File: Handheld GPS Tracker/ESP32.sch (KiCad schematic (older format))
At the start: 27 parts

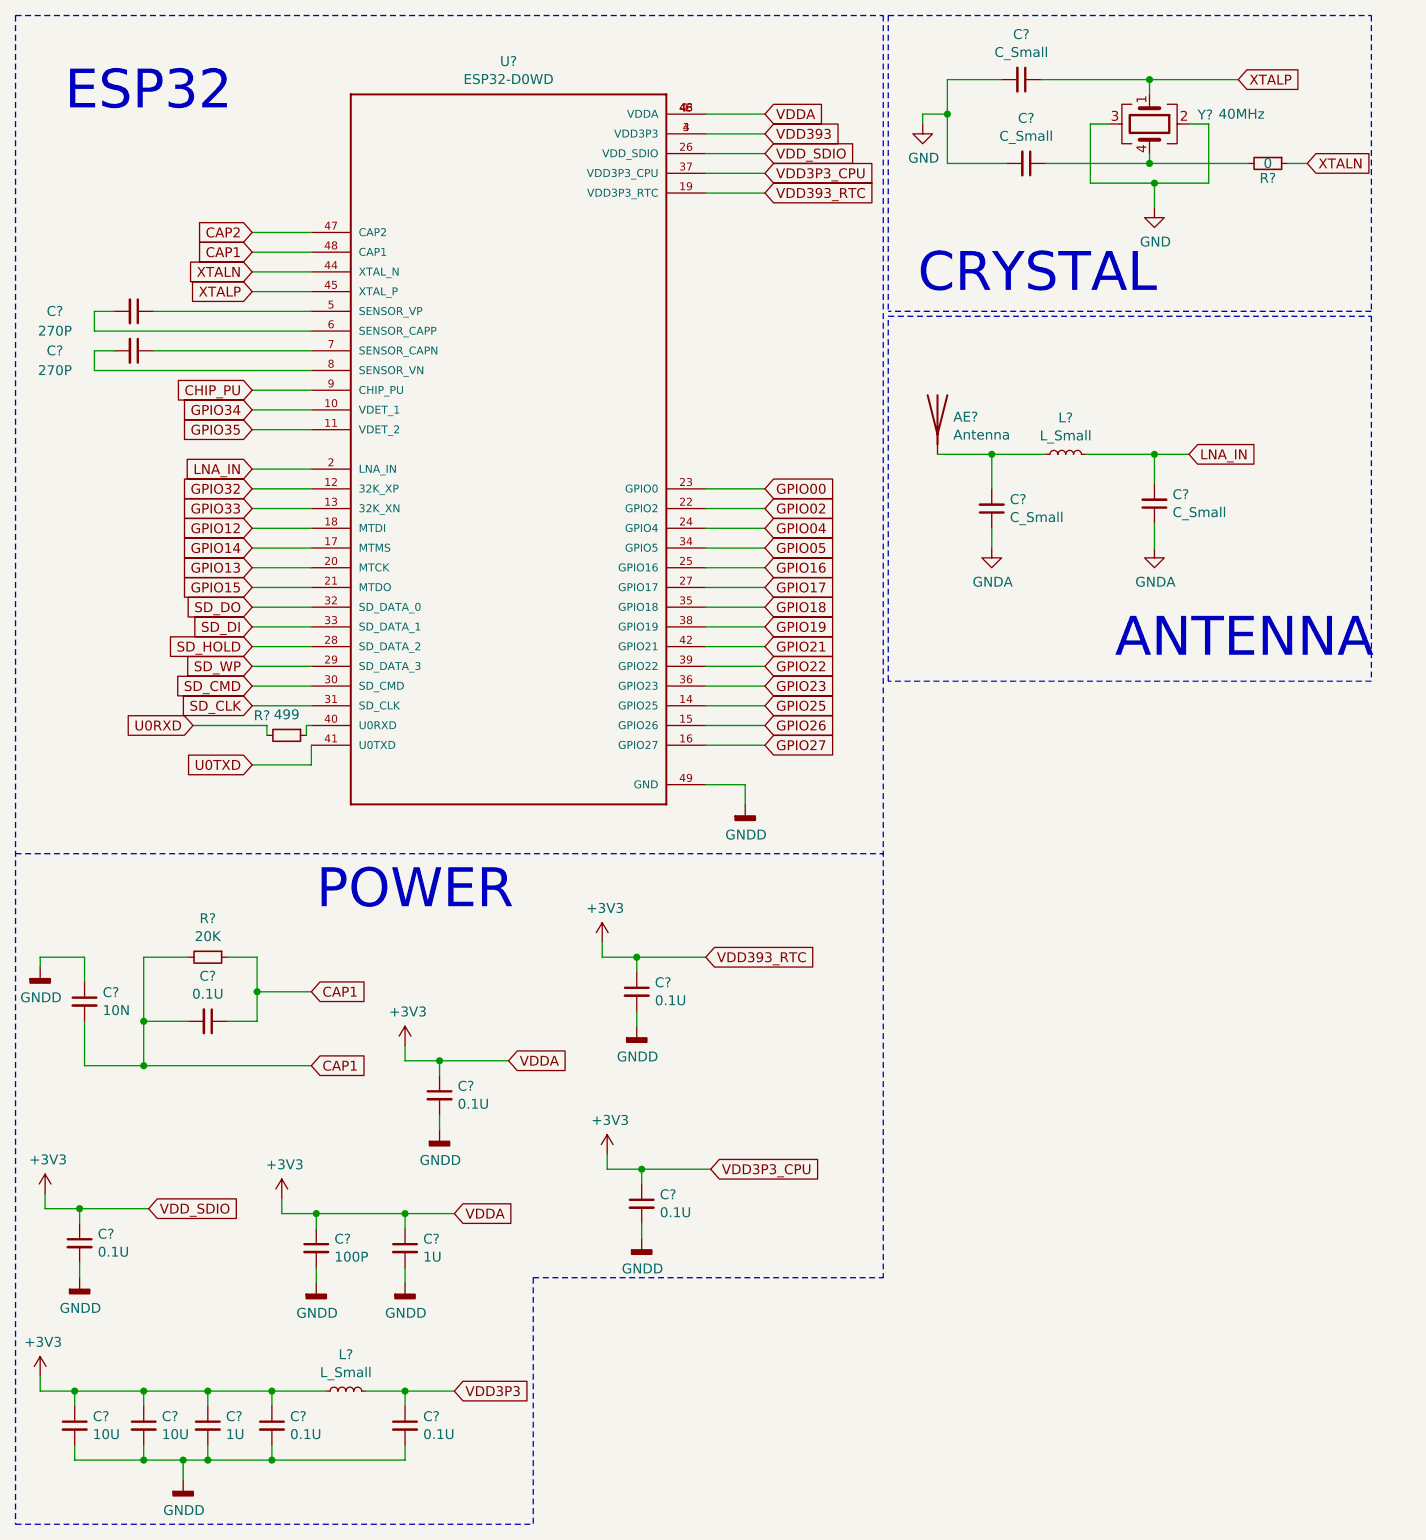
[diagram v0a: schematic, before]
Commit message: Add files via upload
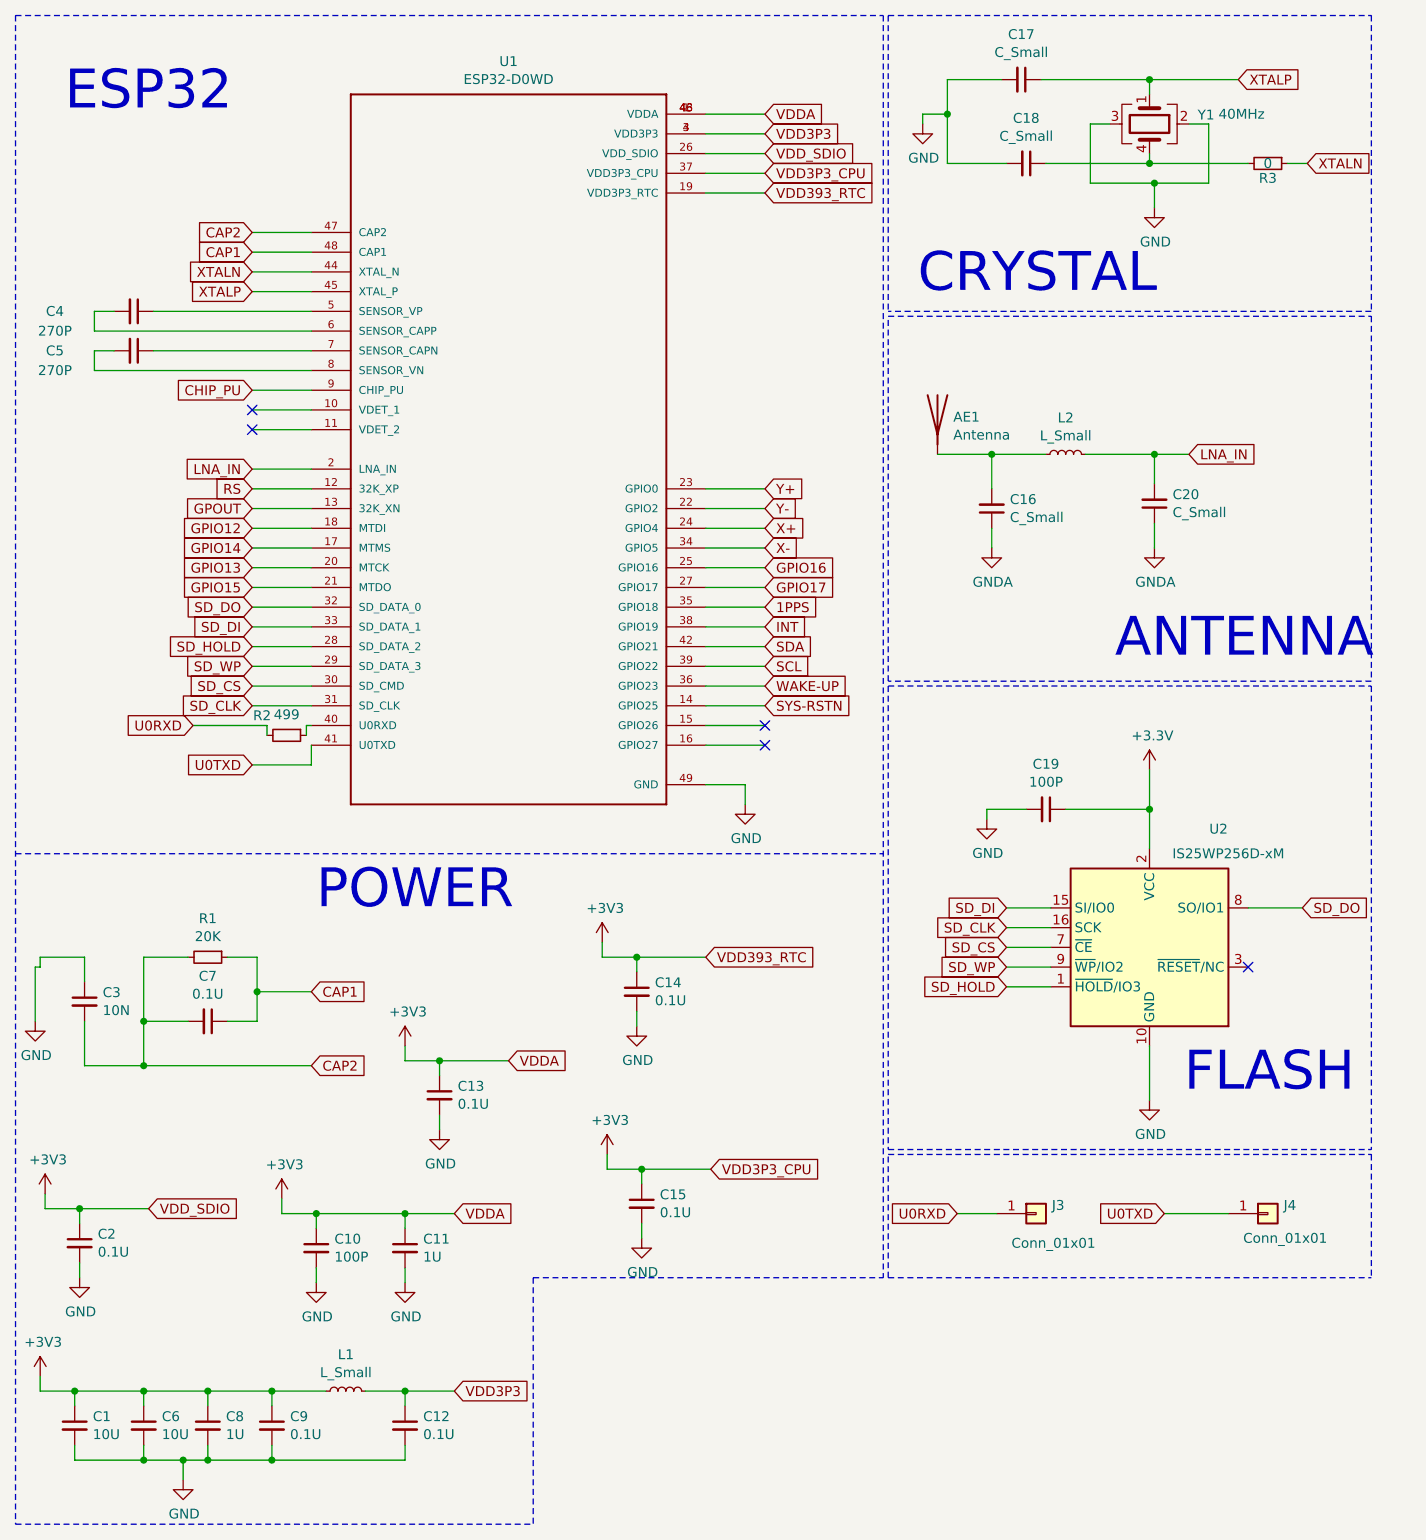
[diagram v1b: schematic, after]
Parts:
- added C19: 100P, symbol Device:C_Small
- added J3, J4: Conn_01x01, symbol Connector_Generic:Conn_01x01
- added U2: IS25WP256D-xM, Package_SO:SOIC-16W_7.5x10.3mm_P1.27mm, symbol Memory_Flash:IS25WP256D-xM
- gave numbers to parts that had none: 27
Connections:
- net GNDD is gone; now on net GND: C1.2, C10.2, C11.2, C12.2, C13.2, C14.2, C15.2, C2.2, C3.1, C6.2, C8.2, C9.2, U1.49 (GND)
- net VDD393 is gone; now on net VDD3P3: U1.3 (VDD3P3), U1.4 (VDD3P3)
- net +3V3: now also C19.1, U2.2 (VCC)
- net CAP1: no longer C3.2, C7.2, R1.2
- net CAP2: now also C3.2, C7.2, R1.2
- net GND: now also C19.2, U2.10 (GND)
- net SD_CLK: now also U2.16 (SCK)
- net SD_DI: now also U2.15 (SI/IO0)
- net SD_DO: now also U2.8 (SO/IO1)
- net SD_HOLD: now also U2.1 (~HOLD~/IO3)
- net SD_WP: now also U2.9 (~WP~/IO2)
- net U0RXD: now also J3.1 (Pin_1)
- net U0TXD: now also J4.1 (Pin_1)
- net GPIO00 renamed Y+
- net GPIO02 renamed Y-
- net GPIO04 renamed X+
- net GPIO05 renamed X-
- net GPIO18 renamed 1PPS
- net GPIO19 renamed INT
- net GPIO21 renamed SDA
- net GPIO22 renamed SCL
- net GPIO23 renamed WAKE-UP
- net GPIO25 renamed SYS-RSTN
- net GPIO26: no longer names the net of U1.15 (GPIO26)
- net GPIO27: no longer names the net of U1.16 (GPIO27)
- net GPIO32 renamed RS
- net GPIO33 renamed GPOUT
- net GPIO34: no longer names the net of U1.10 (VDET_1)
- net GPIO35: no longer names the net of U1.11 (VDET_2)
- net SD_CMD renamed SD_CS
- net SD_CS: now also U2.7 (~CE)
- no-connect marks 0 -> 5
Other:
- note added: "FLASH\n"

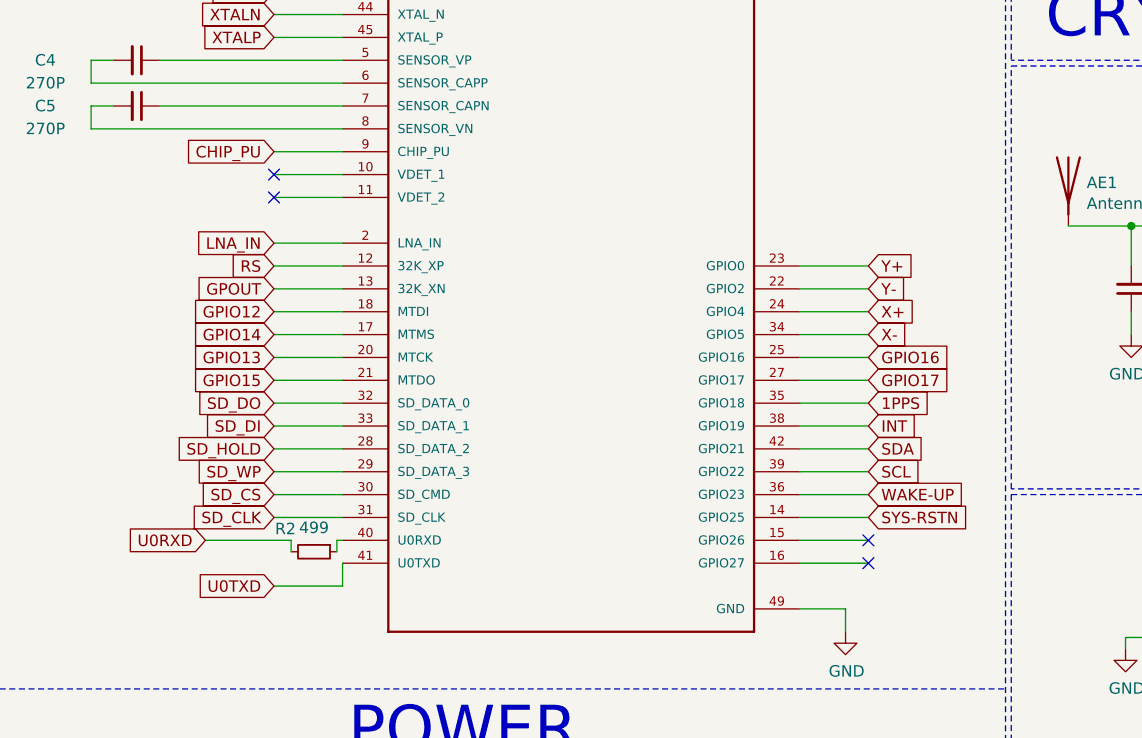
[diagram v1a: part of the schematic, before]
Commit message: Add files via upload
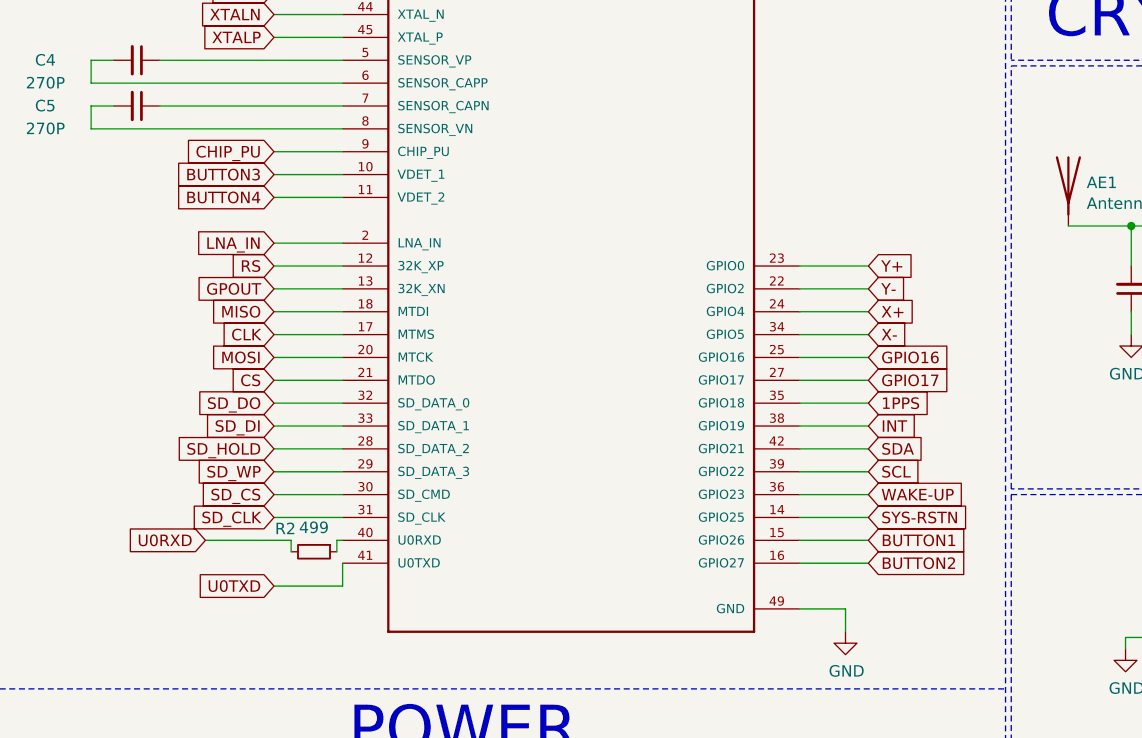
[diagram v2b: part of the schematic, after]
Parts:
- C1, C10, C11, C12, C13, C14, C15, C16, C17, C18, C19, C2, C20, C3, C4, C5, C6, C7, C8, C9: footprint (none) -> Capacitor_SMD:C_0603_1608Metric
- R1, R2, R3: footprint (none) -> Resistor_SMD:R_0402_1005Metric
- U1: footprint QFN35P500X500X90-49N -> ASSETS:QFN35P500X500X90-49N
- Y1: footprint (none) -> Crystal:Crystal_SMD_3225-4Pin_3.2x2.5mm
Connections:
- net BUTTON3: now reaches U1.10 (VDET_1)
- net BUTTON4: now reaches U1.11 (VDET_2)
- net BUTTON1: now reaches U1.15 (GPIO26)
- net BUTTON2: now reaches U1.16 (GPIO27)
- net GPIO12 renamed MISO
- net GPIO13 renamed MOSI
- net GPIO14 renamed CLK
- net GPIO15 renamed CS
- no-connect marks 5 -> 1
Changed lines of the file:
@@
 F 0 "C4" V 1100 1600 50  0000 C CNN
 F 1 "270P" V 1200 1600 50  0000 C CNN
-F 2 "" H 1100 2000 50  0001 C CNN
+F 2 "Capacitor_SMD:C_0603_1608Metric" H 1100 2000 50  0001 C CNN
 F 3 "~" H 1100 2000 50  0001 C CNN
 	1    1100 2000
@@
 F 0 "C5" V 1100 1800 50  0000 C CNN
 F 1 "270P" V 1200 1800 50  0000 C CNN
-F 2 "" H 1100 2200 50  0001 C CNN
+F 2 "Capacitor_SMD:C_0603_1608Metric" H 1100 2200 50  0001 C CNN
 F 3 "~" H 1100 2200 50  0001 C CNN
 	1    1100 2200
@@
 	2000 3100 1700 3100
 Text GLabel 1700 3100 0    50   Input ~ 0
-GPIO12
+MISO
 Wire Wire Line
 	2000 3300 1700 3300
 Text GLabel 1700 3300 0    50   Input ~ 0
-GPIO13
+MOSI
 Wire Wire Line
 	2000 3200 1700 3200
 Text GLabel 1700 3200 0    50   Input ~ 0
-GPIO14
+CLK
 Wire Wire Line
 	2000 3400 1700 3400
 Text GLabel 1700 3400 0    50   Input ~ 0
-GPIO15
+CS
 Wire Wire Line
 	4000 3300 4300 3300
@@
 F 0 "C1" H 892 7696 50  0000 L CNN
 F 1 "10U" H 892 7605 50  0000 L CNN
-F 2 "" H 800 7650 50  0001 C CNN
+F 2 "Capacitor_SMD:C_0603_1608Metric" H 800 7650 50  0001 C CNN
 F 3 "~" H 800 7650 50  0001 C CNN
 	1    800  7650
@@
 F 0 "C6" H 1242 7696 50  0000 L CNN
 F 1 "10U" H 1242 7605 50  0000 L CNN
-F 2 "" H 1150 7650 50  0001 C CNN
+F 2 "Capacitor_SMD:C_0603_1608Metric" H 1150 7650 50  0001 C CNN
 F 3 "~" H 1150 7650 50  0001 C CNN
 	1    1150 7650
@@
 F 0 "C8" H 1567 7696 50  0000 L CNN
 F 1 "1U" H 1567 7605 50  0000 L CNN
-F 2 "" H 1475 7650 50  0001 C CNN
+F 2 "Capacitor_SMD:C_0603_1608Metric" H 1475 7650 50  0001 C CNN
 F 3 "~" H 1475 7650 50  0001 C CNN
 	1    1475 7650
@@
 F 0 "C9" H 1892 7696 50  0000 L CNN
 F 1 "0.1U" H 1892 7605 50  0000 L CNN
-F 2 "" H 1800 7650 50  0001 C CNN
+F 2 "Capacitor_SMD:C_0603_1608Metric" H 1800 7650 50  0001 C CNN
 F 3 "~" H 1800 7650 50  0001 C CNN
 	1    1800 7650
@@
 F 0 "C13" H 2742 6021 50  0000 L CNN
 F 1 "0.1U" H 2742 5930 50  0000 L CNN
-F 2 "" H 2650 5975 50  0001 C CNN
+F 2 "Capacitor_SMD:C_0603_1608Metric" H 2650 5975 50  0001 C CNN
 F 3 "~" H 2650 5975 50  0001 C CNN
 	1    2650 5975
@@
 F 0 "C12" H 2567 7696 50  0000 L CNN
 F 1 "0.1U" H 2567 7605 50  0000 L CNN
-F 2 "" H 2475 7650 50  0001 C CNN
+F 2 "Capacitor_SMD:C_0603_1608Metric" H 2475 7650 50  0001 C CNN
 F 3 "~" H 2475 7650 50  0001 C CNN
 	1    2475 7650
@@
 F 0 "C10" H 2117 6796 50  0000 L CNN
 F 1 "100P" H 2117 6705 50  0000 L CNN
-F 2 "" H 2025 6750 50  0001 C CNN
+F 2 "Capacitor_SMD:C_0603_1608Metric" H 2025 6750 50  0001 C CNN
 F 3 "~" H 2025 6750 50  0001 C CNN
 	1    2025 6750
@@
 F 0 "C11" H 2567 6796 50  0000 L CNN
 F 1 "1U" H 2567 6705 50  0000 L CNN
-F 2 "" H 2475 6750 50  0001 C CNN
+F 2 "Capacitor_SMD:C_0603_1608Metric" H 2475 6750 50  0001 C CNN
 F 3 "~" H 2475 6750 50  0001 C CNN
 	1    2475 6750
@@
 F 0 "C2" H 917 6771 50  0000 L CNN
 F 1 "0.1U" H 917 6680 50  0000 L CNN
-F 2 "" H 825 6725 50  0001 C CNN
+F 2 "Capacitor_SMD:C_0603_1608Metric" H 825 6725 50  0001 C CNN
 F 3 "~" H 825 6725 50  0001 C CNN
 	1    825  6725
@@
 F 0 "C15" H 3767 6571 50  0000 L CNN
 F 1 "0.1U" H 3767 6480 50  0000 L CNN
-F 2 "" H 3675 6525 50  0001 C CNN
+F 2 "Capacitor_SMD:C_0603_1608Metric" H 3675 6525 50  0001 C CNN
 F 3 "~" H 3675 6525 50  0001 C CNN
 	1    3675 6525
@@
 F 0 "C14" H 3742 5496 50  0000 L CNN
 F 1 "0.1U" H 3742 5405 50  0000 L CNN
-F 2 "" H 3650 5450 50  0001 C CNN
+F 2 "Capacitor_SMD:C_0603_1608Metric" H 3650 5450 50  0001 C CNN
 F 3 "~" H 3650 5450 50  0001 C CNN
 	1    3650 5450
@@
 F 0 "R1" V 1279 5275 50  0000 C CNN
 F 1 "20K" V 1370 5275 50  0000 C CNN
-F 2 "" H 1475 5275 50  0001 C CNN
+F 2 "Resistor_SMD:R_0402_1005Metric" H 1475 5275 50  0001 C CNN
 F 3 "~" H 1475 5275 50  0001 C CNN
 	1    1475 5275
@@
 F 0 "C7" V 1246 5600 50  0000 C CNN
 F 1 "0.1U" V 1337 5600 50  0000 C CNN
-F 2 "" H 1475 5600 50  0001 C CNN
+F 2 "Capacitor_SMD:C_0603_1608Metric" H 1475 5600 50  0001 C CNN
 F 3 "~" H 1475 5600 50  0001 C CNN
 	1    1475 5600
@@
 F 0 "C3" H 942 5546 50  0000 L CNN
 F 1 "10N" H 942 5455 50  0000 L CNN
-F 2 "" H 850 5500 50  0001 C CNN
+F 2 "Capacitor_SMD:C_0603_1608Metric" H 850 5500 50  0001 C CNN
 F 3 "~" H 850 5500 50  0001 C CNN
 	1    850  5500
@@
 F 0 "R2" V 1775 4025 50  0000 C CNN
 F 1 "499" V 1770 4150 50  0000 C CNN
-F 2 "" H 1875 4150 50  0001 C CNN
+F 2 "Resistor_SMD:R_0402_1005Metric" H 1875 4150 50  0001 C CNN
 F 3 "~" H 1875 4150 50  0001 C CNN
 	1    1875 4150
@@
 F 0 "Y1" V 6204 1294 50  0000 L CNN
 F 1 "40MHz" V 6200 1400 50  0000 L CNN
-F 2 "" H 6250 1050 50  0001 C CNN
+F 2 "Crystal:Crystal_SMD_3225-4Pin_3.2x2.5mm" H 6250 1050 50  0001 C CNN
 F 3 "~" H 6250 1050 50  0001 C CNN
 	1    6250 1050
@@
 F 0 "C17" V 5371 825 50  0000 C CNN
 F 1 "C_Small" V 5462 825 50  0000 C CNN
-F 2 "" H 5600 825 50  0001 C CNN
+F 2 "Capacitor_SMD:C_0603_1608Metric" H 5600 825 50  0001 C CNN
 F 3 "~" H 5600 825 50  0001 C CNN
 	1    5600 825
@@
 F 0 "C18" V 5396 1250 50  0000 C CNN
 F 1 "C_Small" V 5487 1250 50  0000 C CNN
-F 2 "" H 5625 1250 50  0001 C CNN
+F 2 "Capacitor_SMD:C_0603_1608Metric" H 5625 1250 50  0001 C CNN
 F 3 "~" H 5625 1250 50  0001 C CNN
 	1    5625 1250
@@
 F 0 "R3" V 6925 1250 50  0000 C CNN
 F 1 "0" V 6850 1250 50  0000 C CNN
-F 2 "" H 6850 1250 50  0001 C CNN
+F 2 "Resistor_SMD:R_0402_1005Metric" H 6850 1250 50  0001 C CNN
 F 3 "~" H 6850 1250 50  0001 C CNN
 	1    6850 1250
@@
 F 0 "C16" H 5358 2954 50  0000 R CNN
 F 1 "C_Small" H 5358 3045 50  0000 R CNN
-F 2 "" H 5450 3000 50  0001 C CNN
+F 2 "Capacitor_SMD:C_0603_1608Metric" H 5450 3000 50  0001 C CNN
 F 3 "~" H 5450 3000 50  0001 C CNN
 	1    5450 3000
@@
 F 0 "C20" H 6183 2929 50  0000 R CNN
 F 1 "C_Small" H 6183 3020 50  0000 R CNN
-F 2 "" H 6275 2975 50  0001 C CNN
+F 2 "Capacitor_SMD:C_0603_1608Metric" H 6275 2975 50  0001 C CNN
 F 3 "~" H 6275 2975 50  0001 C CNN
 	1    6275 2975
@@
 F 0 "C19" V 5496 4525 50  0000 C CNN
 F 1 "100P" V 5587 4525 50  0000 C CNN
-F 2 "" H 5725 4525 50  0001 C CNN
+F 2 "Capacitor_SMD:C_0603_1608Metric" H 5725 4525 50  0001 C CNN
 F 3 "~" H 5725 4525 50  0001 C CNN
 	1    5725 4525
@@
 F 0 "U1" H 3000 4667 50  0000 C CNN
 F 1 "ESP32-D0WD" H 3000 4576 50  0000 C CNN
-F 2 "QFN35P500X500X90-49N" H 3000 2700 50  0001 L BNN
+F 2 "ASSETS:QFN35P500X500X90-49N" H 3000 2700 50  0001 L BNN
 F 3 "1.7" H 3000 2700 50  0001 L BNN
 F 4 "QFN-48" H 3000 2700 50  0001 L BNN "Field4"
@@
 Text GLabel 4300 3900 2    50   Input ~ 0
 WAKE-UP
-NoConn ~ 4300 4200
-NoConn ~ 1700 2500
-NoConn ~ 1700 2600
-NoConn ~ 4300 4100
 Text GLabel 4300 3400 2    50   Input ~ 0
 GPIO17
@@
 Text GLabel 1700 3000 0    50   Input ~ 0
 GPOUT
+Text GLabel 4300 4100 2    50   Input ~ 0
+BUTTON1
+Text GLabel 4300 4200 2    50   Input ~ 0
+BUTTON2
+Text GLabel 1700 2500 0    50   Input ~ 0
+BUTTON3
+Text GLabel 1700 2600 0    50   Input ~ 0
+BUTTON4
 $EndSCHEMATC
